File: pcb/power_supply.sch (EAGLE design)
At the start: 33 parts, among them U1 RASPBERRY_PI_3_MODEL_B+, U10 2DD2652-7, U11 TI_NATIONAL_SEMICONDUCTOR_LM1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, U2 LM1085IT-5.0, U3 2DD2652-7, U4 2DD2652-7, U5 2DD2652-7, U6 2DD2652-7, U7 2DD2652-7, U8 2DD2652-7, U9 2DD2652-7, X1 MKKDS02, X2 MKKDS02, X3 MKKDS02, X4 MKKDS02, X5 MKKDS02, X6 FC681478FC681478, X7 MKDSN1,5/2-5,08

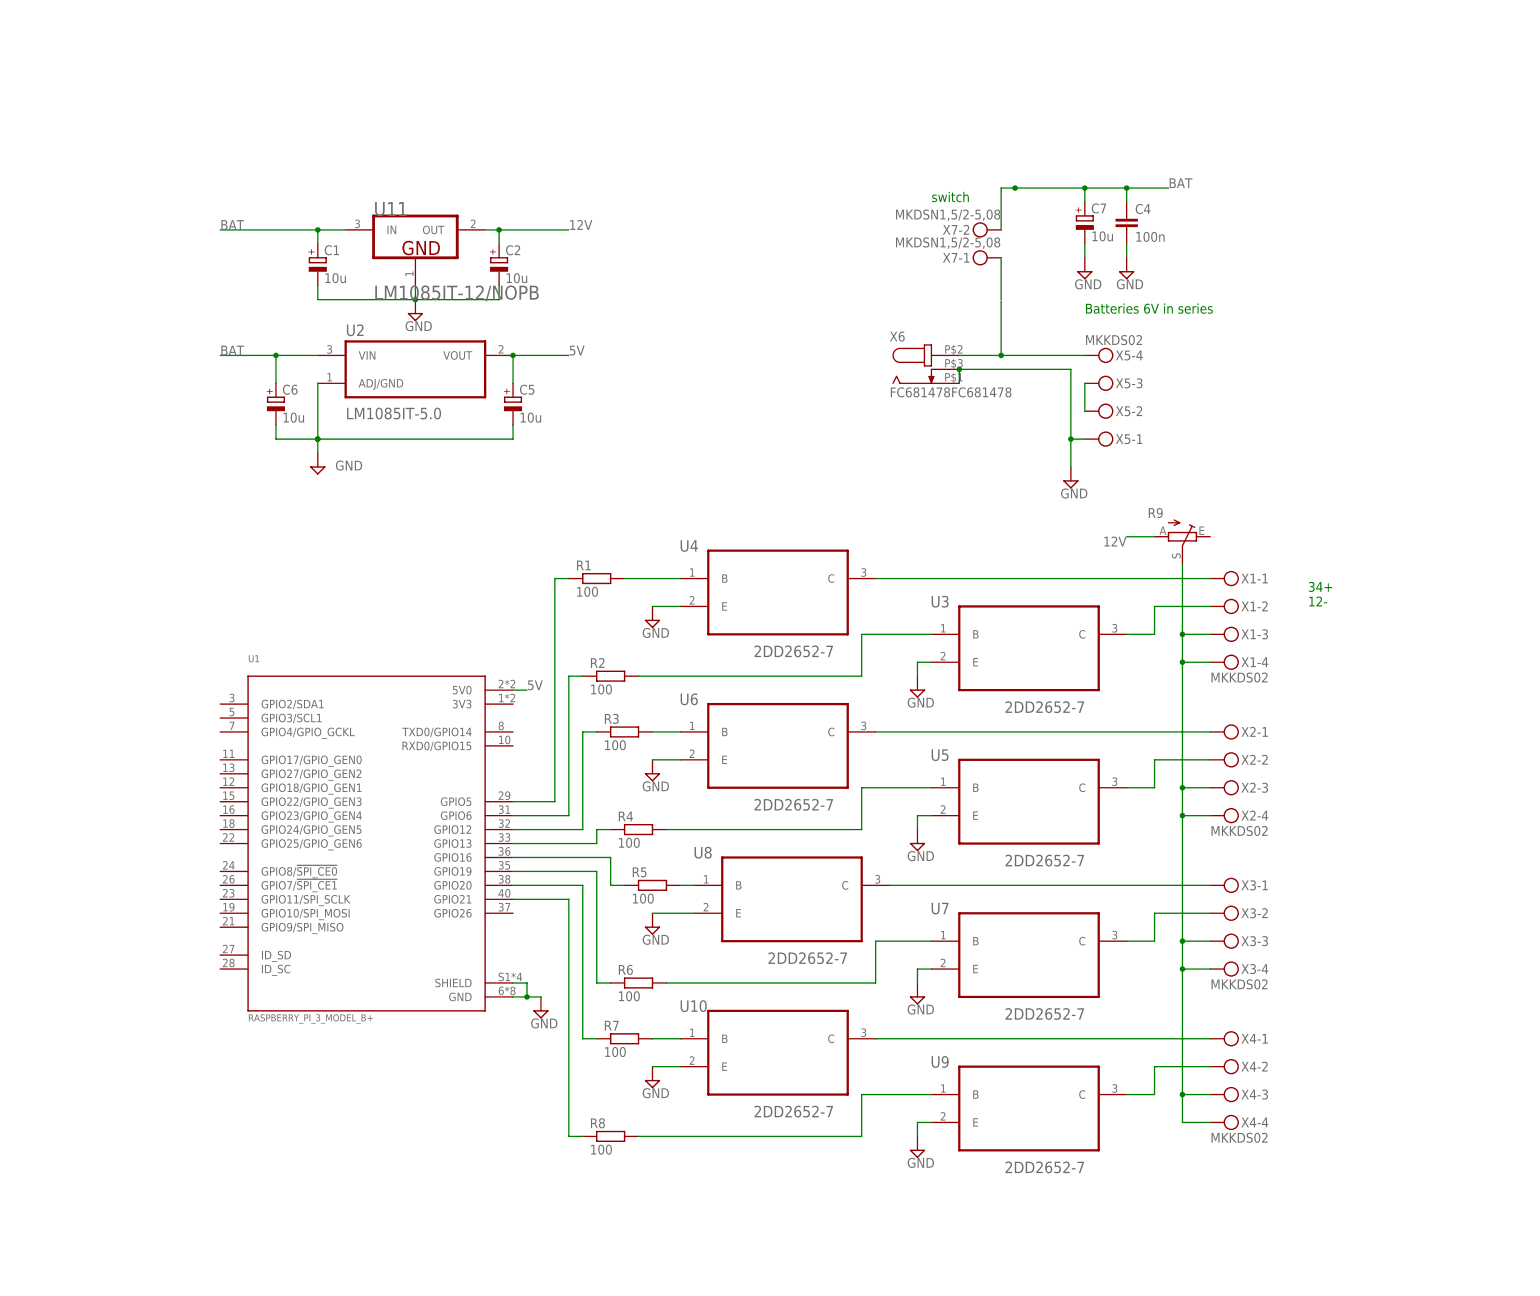
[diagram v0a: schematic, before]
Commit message: pcb - schematic done for now
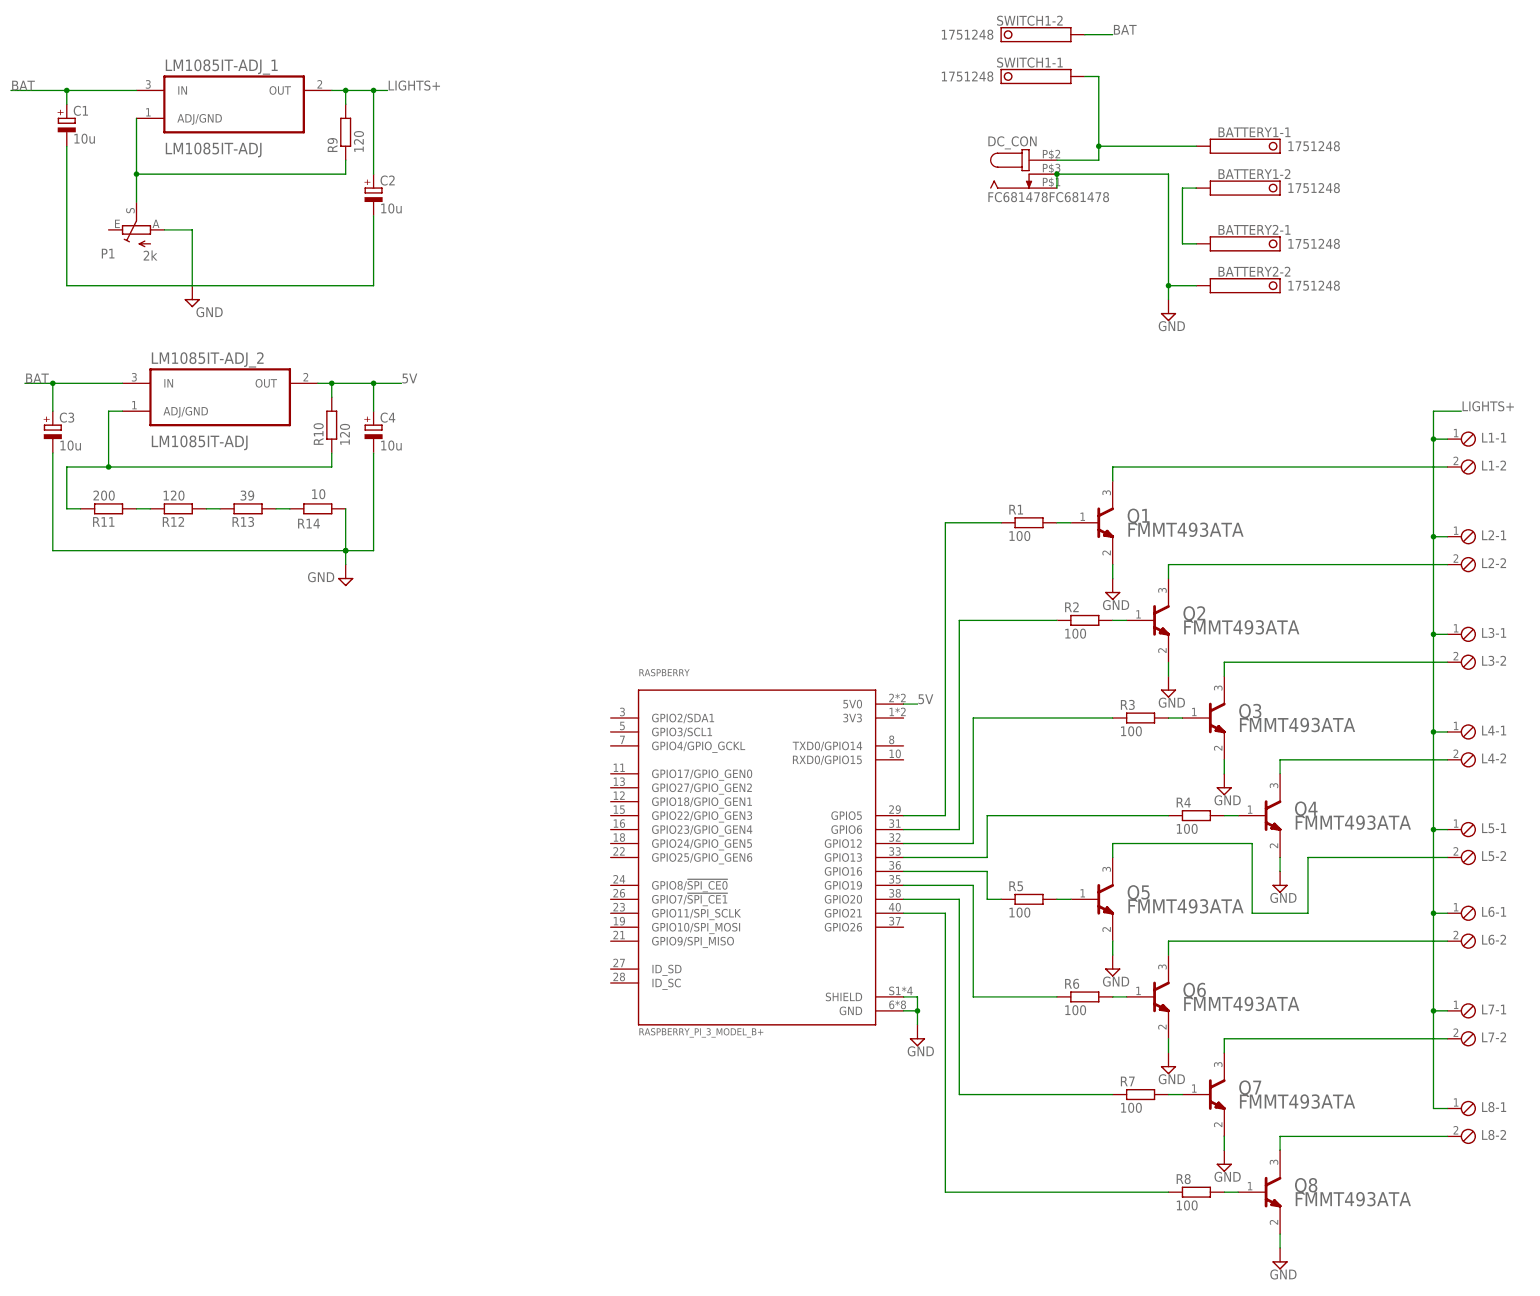
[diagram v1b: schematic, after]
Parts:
- removed C5, C6, C7: 10u, rcl:CPOL-EUB/3528-21R
- removed U1: RASPBERRY_PI_3_MODEL_B+, RASPBERRY_PI_3_MODEL_B_:RASPBERRY_PI_3_MODEL_B+
- removed U10, U3, U4, U5, U6, U7, U8, U9: 2DD2652-7, 2DD2652-7:2DD2652-7
- removed U11: TI_NATIONAL_SEMICONDUCTOR_LM1085IT-12-NOPBTI_NATIONAL_SEMIC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, LM1085IT-12:TI_NATIONAL_SEMICONDUCTOR_LM1085IT-12-NOPBTI_NATIONAL_SEMICONDUCTOR_LM1085IT-12-NOPB_0_0
- removed U2: LM1085IT-5.0, LM1085IT-5.0:LM1085IT-5.0
- removed X1, X2, X3, X4, X5: MKKDS02, con-phoenix-508:MKKDS02
- removed X6: FC681478FC681478, FC681478:FC681478FC681478
- removed X7: MKDSN1,5/2-5,08, con-phoenix-508:MKDSN1,5/2-5,08
- added BATTERY1, BATTERY2, SWITCH1: 1751248, con-phoenix-350:1751248
- added C3: 10u, rcl:CPOL-EUB/3528-21R
- added DC_CON: FC681478FC681478, FC681478:FC681478FC681478
- added L1, L2, L3, L4, L5, L6, L7, L8: (no value), con-phoenix-254:MPT2
- added LM1085IT-ADJ_1, LM1085IT-ADJ_2: LM1085IT-ADJ, LM1085IT-ADJ:LM1085IT-ADJ
- added P1: 2k, pot:TRIM_EU-CA6V
- added Q1, Q2, Q3, Q4, Q5, Q6, Q7, Q8: DIODES_FMMT493ATADIODES_FMMT493ATA_0_0, Diodes - FMMT493ATA:DIODES_FMMT493ATADIODES_FMMT493ATA_0_0
- added R10, R12: 120, rcl:R-EU_R0805
- added R11: 200, rcl:R-EU_R0805
- added R13: 39, rcl:R-EU_R0805
- added R14: 10, rcl:R-EU_R0805
- added RASPBERRY: RASPBERRY_PI_3_MODEL_B+, RASPBERRY_PI_3_MODEL_B_:RASPBERRY_PI_3_MODEL_B+
- C4: value 100n -> 10u; device rcl:C-EUC0805 -> rcl:CPOL-EUB/3528-21R
- R9: value (none) -> 120; device pot:TRIM_EU-CA6V -> rcl:R-EU_R0805
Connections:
- removed net 12V: C2.+, R9.A, U11.OUT
- removed net N$28: X7-1.KL
- new net N$2: LM1085IT-ADJ_2.ADJ/GND, R10.1, R11.2
- new net N$29: LM1085IT-ADJ_1.ADJ/GND, P1.S, R9.1
- new net N$30: R11.1, R12.2
- new net N$31: R12.1, R13.2
- new net N$32: R13.1, R14.1
- net 5V: now also C4.+, LM1085IT-ADJ_2.OUT, R10.2, RASPBERRY.5V0; no longer C5.+, U1.5V0, U2.VOUT
- net BAT: now also C3.+, LM1085IT-ADJ_1.IN, LM1085IT-ADJ_2.IN, SWITCH1-2.K; no longer C4.1, C6.+, C7.+, U11.IN, U2.VIN, X7-2.KL
- net GND: now also BATTERY2-2.K, C3.-, C4.-, DC_CON.1, DC_CON.2, P1.A, Q1.E, Q2.E, Q3.E, Q4.E, Q5.E, Q6.E, Q7.E, Q8.E, R14.2, RASPBERRY.GND, RASPBERRY.SHIELD; no longer C4.2, C5.-, C6.-, C7.-, U1.GND, U1.SHIELD, U10.E, U11.GND, U2.ADJ/GND, U3.E, U4.E, U5.E, U6.E, U7.E, U8.E, U9.E, X5-1.KL, X6.1, X6.2
- net LIGHTS+: now also C2.+, L1-1.1, L2-1.1, L3-1.1, L4-1.1, L5-1.1, L6-1.1, L7-1.1, L8-1.1, LM1085IT-ADJ_1.OUT, R9.2; no longer R9.S, X1-3.KL, X1-4.KL, X2-3.KL, X2-4.KL, X3-3.KL, X3-4.KL, X4-3.KL, X4-4.KL
- net N$1: now also L1-2.1, Q1.C; no longer U4.C, X1-1.KL
- net N$10: now also L4-2.1, Q4.C; no longer U6.C, X2-1.KL
- net N$11: now also Q5.B, R5.2; no longer R4.2, U5.B
- net N$12: now also L5-2.1, Q5.C; no longer U8.C, X3-1.KL
- net N$13: now also Q6.B, R6.2; no longer U10.C, X4-1.KL
- net N$14: now also L6-2.1, Q6.C; no longer U5.C, X2-2.KL
- net N$15: now also Q7.B, R7.2; no longer U7.C, X3-2.KL
- net N$16: now also L7-2.1, Q7.C; no longer U9.C, X4-2.KL
- net N$17: now also Q8.B, R8.2; no longer R3.1, U1.GPIO12
- net N$18: now also L8-2.1, Q8.C; no longer R7.1, U1.GPIO20
- net N$19: now also R1.1, RASPBERRY.GPIO5; no longer R5.1, U1.GPIO16
- net N$20: now also R2.1, RASPBERRY.GPIO6; no longer R6.2, U7.B
- net N$21: now also R3.1, RASPBERRY.GPIO12; no longer R2.1, U1.GPIO6
- net N$22: now also Q1.B; no longer U4.B
- net N$23: now also RASPBERRY.GPIO13; no longer U1.GPIO13
- net N$24: now also R5.1, RASPBERRY.GPIO16; no longer R3.2, U6.B
- net N$25: now also R6.1, RASPBERRY.GPIO19; no longer R8.2, U9.B
- net N$26: now also R7.1, RASPBERRY.GPIO20; no longer R5.2, U8.B
- net N$27: now also R8.1, RASPBERRY.GPIO21; no longer R7.2, U10.B
- net N$3: now also BATTERY1-1.K, DC_CON.3, SWITCH1-1.K; no longer X5-4.KL, X6.3
- net N$4: now also BATTERY1-2.K, BATTERY2-1.K; no longer X5-2.KL, X5-3.KL
- net N$5: now also Q2.B, R2.2; no longer R1.1, U1.GPIO5
- net N$6: now also L2-2.1, Q2.C; no longer R2.2, U3.B
- net N$7: now also Q3.B, R3.2; no longer R6.1, U1.GPIO19
- net N$8: now also L3-2.1, Q3.C; no longer U3.C, X1-2.KL
- net N$9: now also Q4.B, R4.2; no longer R8.1, U1.GPIO21
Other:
- note removed: "34+ 12-"
- note removed: "Batteries 6V in series"
- note removed: "switch"
- moved on the sheet: C1, C2, R1, R2, R3, R4, R5, R6, R7, R8
